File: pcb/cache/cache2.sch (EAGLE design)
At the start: 14 parts

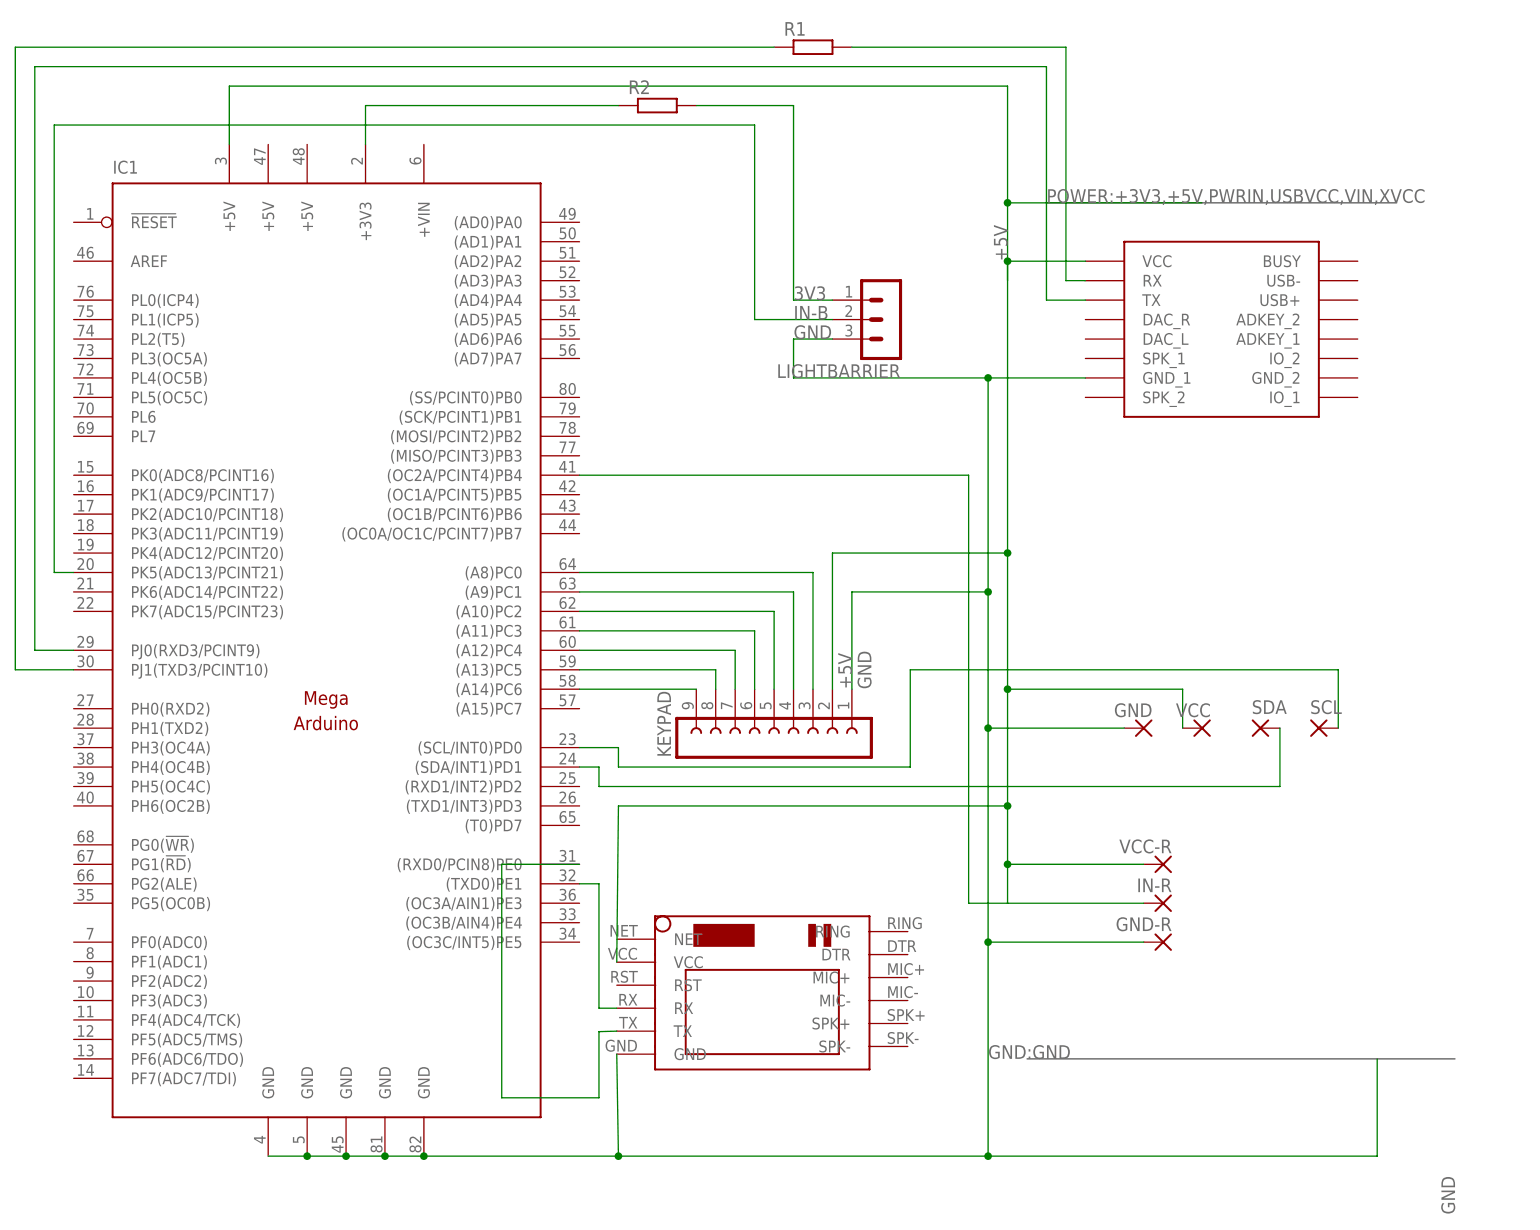
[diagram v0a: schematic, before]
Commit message: updated pcb
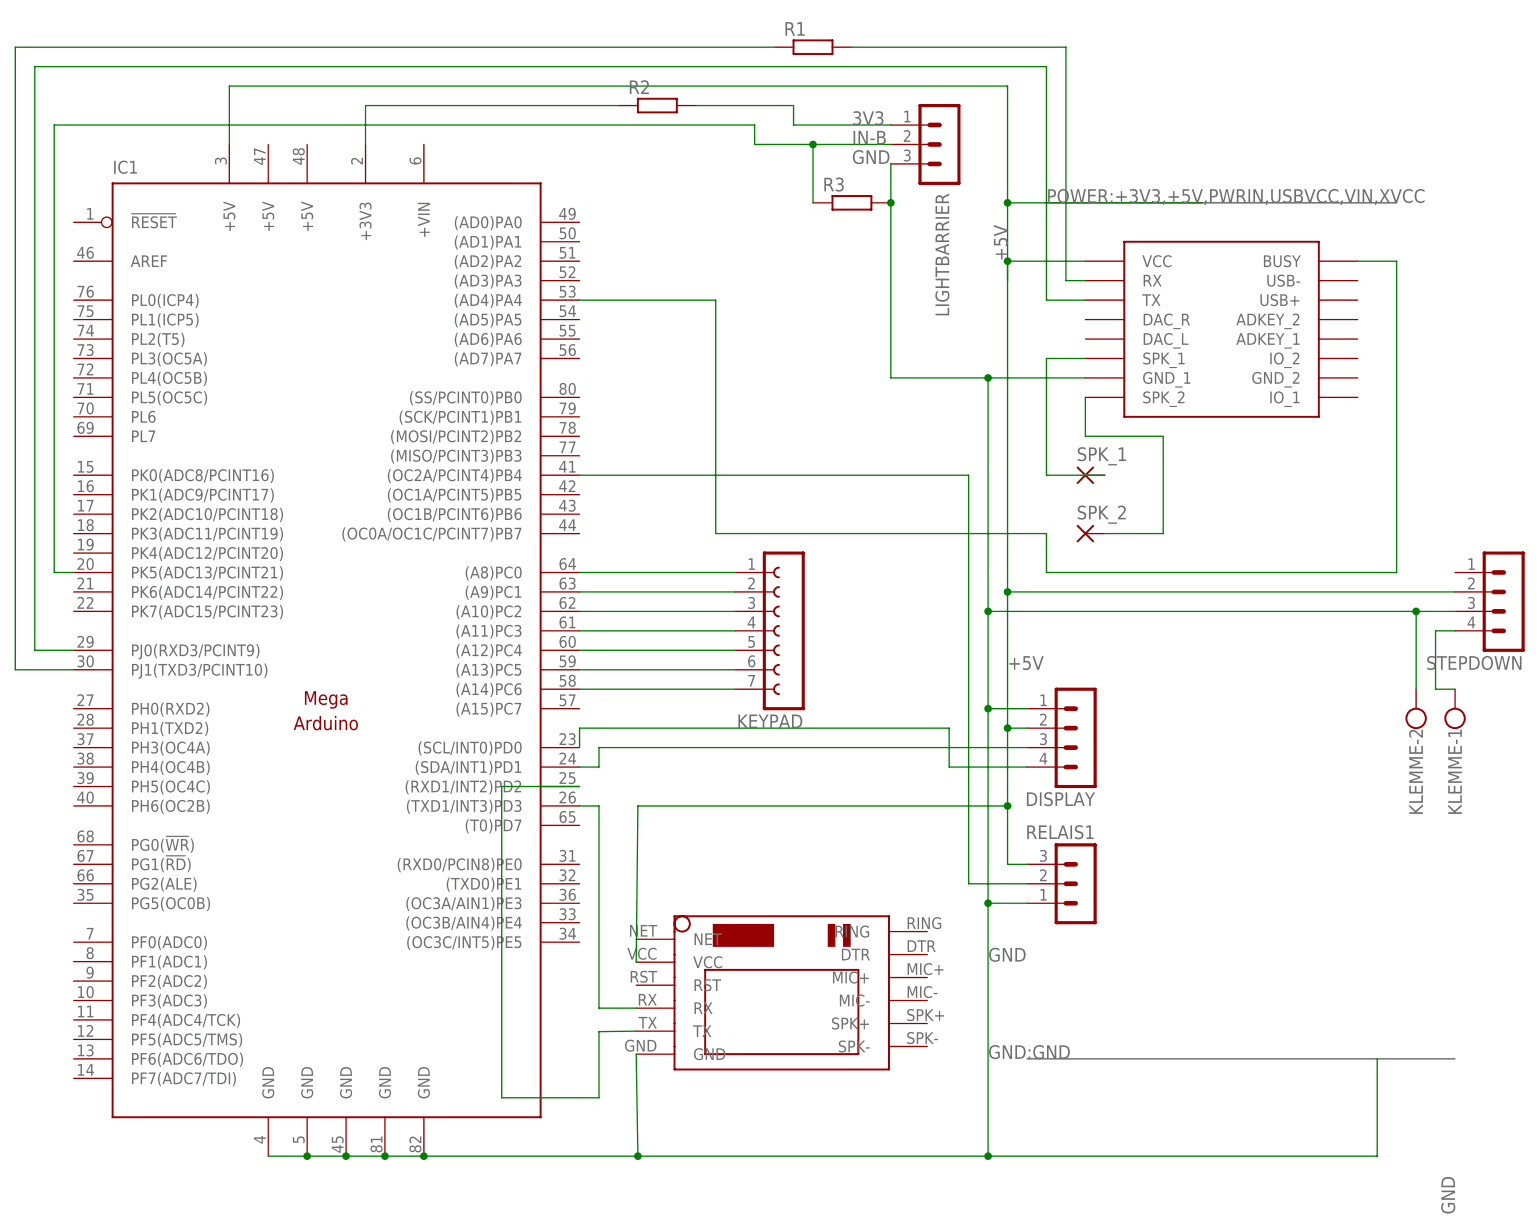
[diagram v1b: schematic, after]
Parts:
- removed GND, GND-R, IN-R, SCL, SDA, VCC, VCC-R: (no value), wirepad:1,6/0,8
- added DISPLAY, STEPDOWN: (no value), con-lstb:MA04-1
- added KLEMME: (no value), con-wago-500:W237-102
- added R3: (no value), rcl:R-EU_0204/7
- added RELAIS1: (no value), con-lstb:MA03-1
- added SPK_1, SPK_2: (no value), wirepad:1,6/0,8
- KEYPAD: device con-lsta:FE09-1 -> con-lsta:FE07-1
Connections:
- new net IN+: KLEMME-1.KL, STEPDOWN.4
- new net N$17: SPK_2.P, U$1.SPK_2
- new net N$18: SPK_1.P, U$1.SPK_1
- new net N$19: IC1.(AD4)PA4, U$1.BUSY
- net +5V: now also DISPLAY.2, RELAIS1.3, STEPDOWN.2; no longer KEYPAD.2, VCC-R.P, VCC.P
- net GND: now also DISPLAY.1, KLEMME-2.KL, R3.2, RELAIS1.1, STEPDOWN.3; no longer GND-R.P, GND.P, KEYPAD.1
- net IN-B: now also R3.1
- net N$1: now also IC1.(RXD1/INT2)PD2; no longer IC1.(RXD0/PCIN8)PE0
- net N$10: now also KEYPAD.3; no longer KEYPAD.5
- net N$11: now also KEYPAD.2; no longer KEYPAD.4
- net N$12: now also KEYPAD.1; no longer KEYPAD.3
- net N$2: now also IC1.(TXD1/INT3)PD3; no longer IC1.(TXD0)PE1
- net N$3: now also RELAIS1.2; no longer IN-R.P
- net N$4: now also DISPLAY.3; no longer SDA.P
- net N$5: now also DISPLAY.4; no longer SCL.P
- net N$6: now also KEYPAD.7; no longer KEYPAD.9
- net N$7: now also KEYPAD.6; no longer KEYPAD.8
- net N$8: now also KEYPAD.5; no longer KEYPAD.7
- net N$9: now also KEYPAD.4; no longer KEYPAD.6
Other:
- moved on the sheet: LIGHTBARRIER
